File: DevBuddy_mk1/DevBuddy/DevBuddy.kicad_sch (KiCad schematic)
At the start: 5 parts, among them U1 RP2354B

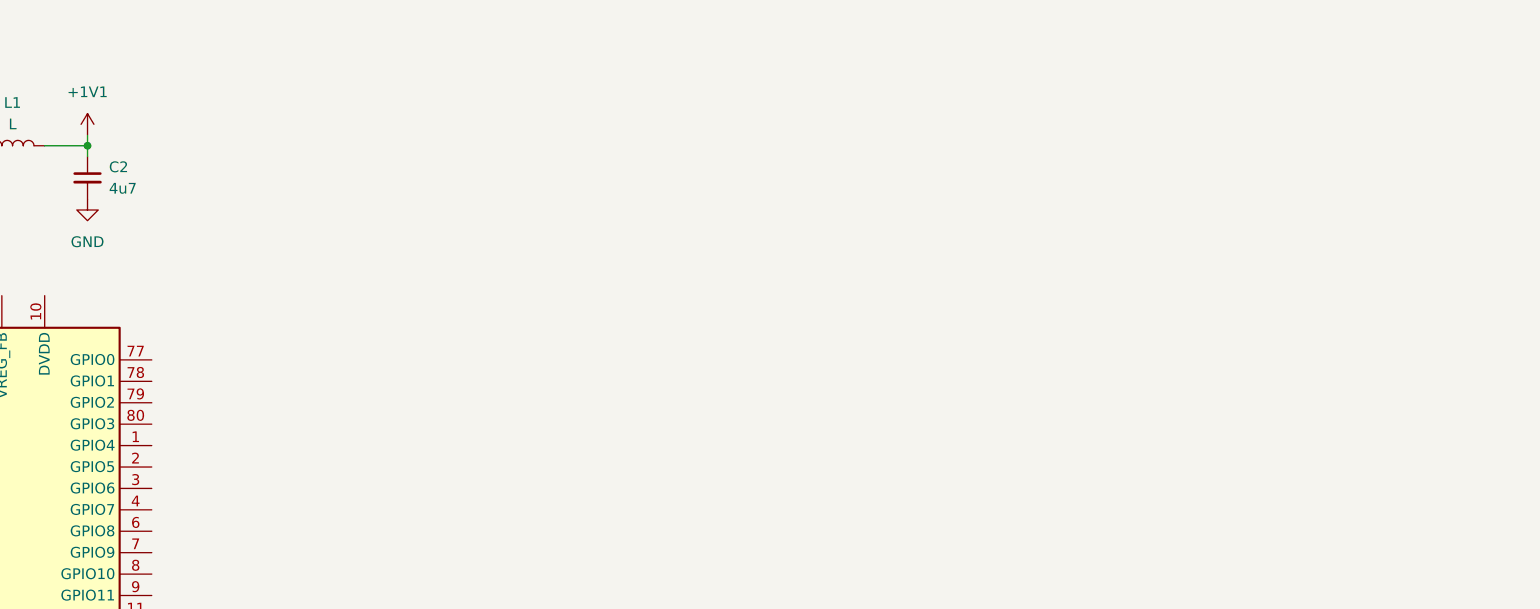
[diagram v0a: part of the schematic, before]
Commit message: Hardware changes, ADC and start of power.
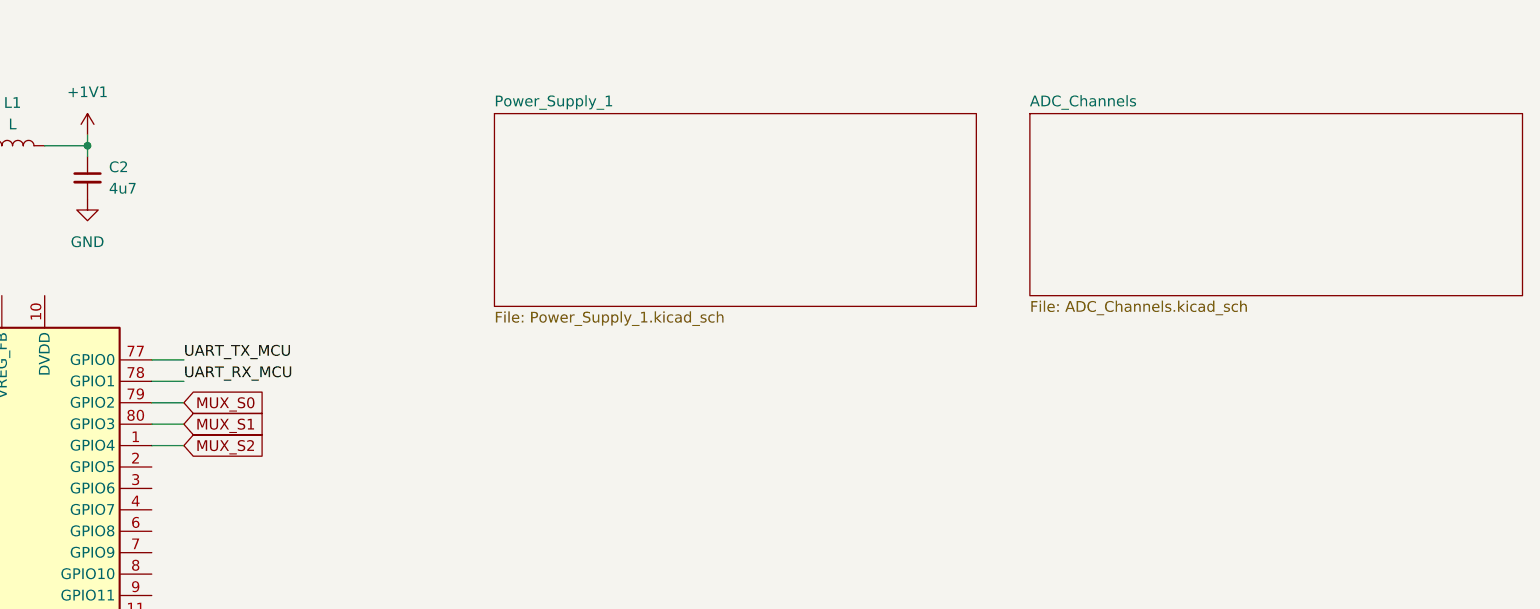
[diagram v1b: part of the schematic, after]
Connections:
- net MUX_S2: now reaches U1.1 (GPIO4)
- net UART_TX_MCU: now reaches U1.77 (GPIO0)
- net UART_RX_MCU: now reaches U1.78 (GPIO1)
- net MUX_S0: now reaches U1.79 (GPIO2)
- net MUX_S1: now reaches U1.80 (GPIO3)
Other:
- added sheet ADC_Channels (ADC_Channels.kicad_sch)
- added sheet Power_Supply_1 (Power_Supply_1.kicad_sch)
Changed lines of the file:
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@@
+	(wire
+		(pts
+			(xy 144.78 71.12) (xy 148.59 71.12)
+		)
+		(stroke
+			(width 0)
+			(type default)
+		)
+	)
 	(wire
 		(pts
@@
 	(wire
 		(pts
+			(xy 144.78 76.2) (xy 148.59 76.2)
+		)
+		(stroke
+			(width 0)
+			(type default)
+		)
+	)
+	(wire
+		(pts
+			(xy 144.78 81.28) (xy 148.59 81.28)
+		)
+		(stroke
+			(width 0)
+			(type default)
+		)
+	)
+	(wire
+		(pts
 			(xy 137.16 45.72) (xy 137.16 46.99)
 		)
@@
 	(wire
 		(pts
+			(xy 144.78 78.74) (xy 148.59 78.74)
+		)
+		(stroke
+			(width 0)
+			(type default)
+		)
+	)
+	(wire
+		(pts
+			(xy 144.78 73.66) (xy 148.59 73.66)
+		)
+		(stroke
+			(width 0)
+			(type default)
+		)
+	)
+	(wire
+		(pts
 			(xy 76.2 44.45) (xy 60.96 44.45)
 		)
@@
 			(width 0)
 			(type default)
+		)
+	)
+	(label "UART_RX_MCU"
+		(at 148.59 73.66 0)
+		(effects
+			(font
+				(size 1.27 1.27)
+			)
+			(justify left bottom)
+		)
+	)
+	(label "UART_TX_MCU"
+		(at 148.59 71.12 0)
+		(effects
+			(font
+				(size 1.27 1.27)
+			)
+			(justify left bottom)
+		)
+	)
+	(global_label "MUX_S1"
+		(shape input)
+		(at 148.59 78.74 0)
+		(fields_autoplaced yes)
+		(effects
+			(font
+				(size 1.27 1.27)
+			)
+			(justify left)
+		)
+		(property "Intersheetrefs" "${INTERSHEET_REFS}"
+			(at 158.9532 78.74 0)
+			(effects
+				(font
+					(size 1.27 1.27)
+				)
+				(justify left)
+				(hide yes)
+			)
+		)
+	)
+	(global_label "MUX_S2"
+		(shape input)
+		(at 148.59 81.28 0)
+		(fields_autoplaced yes)
+		(effects
+			(font
+				(size 1.27 1.27)
+			)
+			(justify left)
+		)
+		(property "Intersheetrefs" "${INTERSHEET_REFS}"
+			(at 158.9532 81.28 0)
+			(effects
+				(font
+					(size 1.27 1.27)
+				)
+				(justify left)
+				(hide yes)
+			)
+		)
+	)
+	(global_label "MUX_S0"
+		(shape input)
+		(at 148.59 76.2 0)
+		(fields_autoplaced yes)
+		(effects
+			(font
+				(size 1.27 1.27)
+			)
+			(justify left)
+		)
+		(property "Intersheetrefs" "${INTERSHEET_REFS}"
+			(at 158.9532 76.2 0)
+			(effects
+				(font
+					(size 1.27 1.27)
+				)
+				(justify left)
+				(hide yes)
+			)
 		)
 	)
@@
 				)
 			)
+		)
+	)
+	(sheet
+		(at 185.42 41.91)
+		(size 57.15 22.86)
+		(exclude_from_sim no)
+		(in_bom yes)
+		(on_board yes)
+		(dnp no)
+		(fields_autoplaced yes)
+		(stroke
+			(width 0.1524)
+			(type solid)
+		)
+		(fill
+			(color 0 0 0 0.0000)
+		)
+		(property "Sheetname" "Power_Supply_1"
+			(at 185.42 41.1984 0)
+			(effects
+				(font
+					(size 1.27 1.27)
+				)
+				(justify left bottom)
+			)
+		)
+		(property "Sheetfile" "Power_Supply_1.kicad_sch"
+			(at 185.42 65.3546 0)
+			(effects
+				(font
+					(size 1.27 1.27)
+				)
+				(justify left top)
+			)
+		)
+		(instances
+			(project "DevBuddy"
+				(path "/cd44a09a-8e2e-49d9-bb56-7efc0bfafbd6"
+					(page "2")
+				)
+			)
+		)
+	)
+	(sheet
+		(at 248.92 41.91)
+		(size 58.42 21.59)
+		(exclude_from_sim no)
+		(in_bom yes)
+		(on_board yes)
+		(dnp no)
+		(fields_autoplaced yes)
+		(stroke
+			(width 0.1524)
+			(type solid)
+		)
+		(fill
+			(color 0 0 0 0.0000)
+		)
+		(property "Sheetname" "ADC_Channels"
+			(at 248.92 41.1984 0)
+			(effects
+				(font
+					(size 1.27 1.27)
+				)
+				(justify left bottom)
+			)
+		)
+		(property "Sheetfile" "ADC_Channels.kicad_sch"
+			(at 248.92 64.0846 0)
+			(effects
+				(font
+					(size 1.27 1.27)
+				)
+				(justify left top)
+			)
+		)
+		(instances
+			(project "DevBuddy"
+				(path "/cd44a09a-8e2e-49d9-bb56-7efc0bfafbd6"
+					(page "3")
+				)
+			)
